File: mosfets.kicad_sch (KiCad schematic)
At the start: 35 parts, among them Q10 IXTP90N15T, Q11 IXTP90N15T, Q12 IXTP90N15T, Q13 IXTP90N15T, U10 IRS21867S, U6 IRS21867S, U7 IR2110, U9 IRS21867S

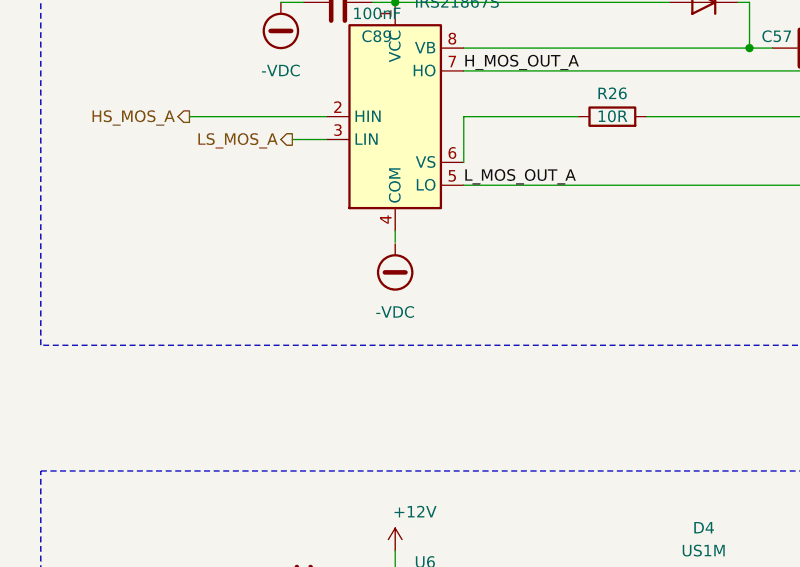
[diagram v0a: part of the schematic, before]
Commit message: MD DONE IHOPE
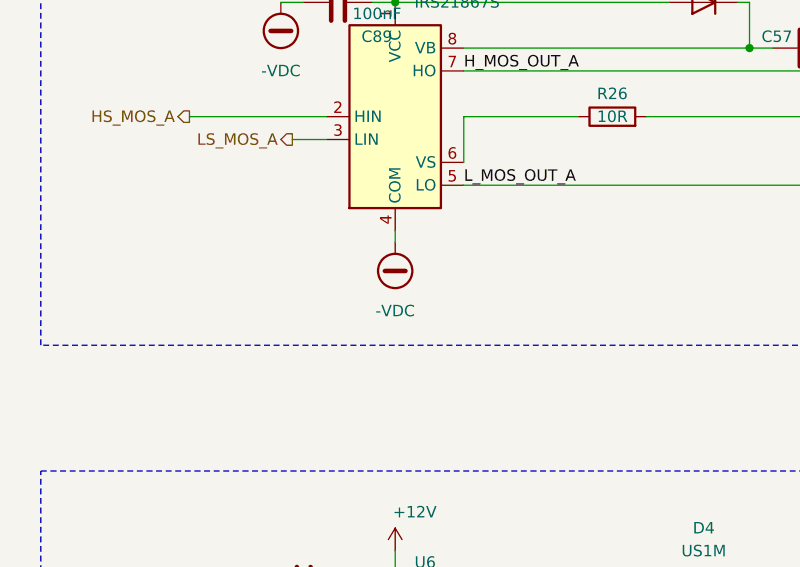
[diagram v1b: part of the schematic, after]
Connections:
- net -VDC: now also U9.4 (COM)
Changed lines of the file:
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@@
 	(symbol
 		(lib_id "power:-VDC")
-		(at 53.34 52.2329 180)
+		(at 53.34 52.07 180)
 		(unit 1)
 		(exclude_from_sim no)
@@
 		(fields_autoplaced yes)
 		(property "Reference" "#PWR0101"
-			(at 53.34 49.6929 0)
+			(at 53.34 49.53 0)
 			(effects
 				(font
@@
 		)
 		(property "Value" "-VDC"
-			(at 53.34 59.8529 0)
+			(at 53.34 59.69 0)
 			(effects
 				(font
@@
 		)
 		(property "Footprint" ""
-			(at 53.34 52.2329 0)
+			(at 53.34 52.07 0)
 			(effects
 				(font
@@
 		)
 		(property "Datasheet" ""
-			(at 53.34 52.2329 0)
+			(at 53.34 52.07 0)
 			(effects
 				(font
@@
 		)
 		(property "Description" "Power symbol creates a global label with name \"-VDC\""
-			(at 53.34 52.2329 0)
+			(at 53.34 52.07 0)
 			(effects
 				(font
